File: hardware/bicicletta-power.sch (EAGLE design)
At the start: 23 parts, among them IC1 LM5017, IC2 LM1117-3.3

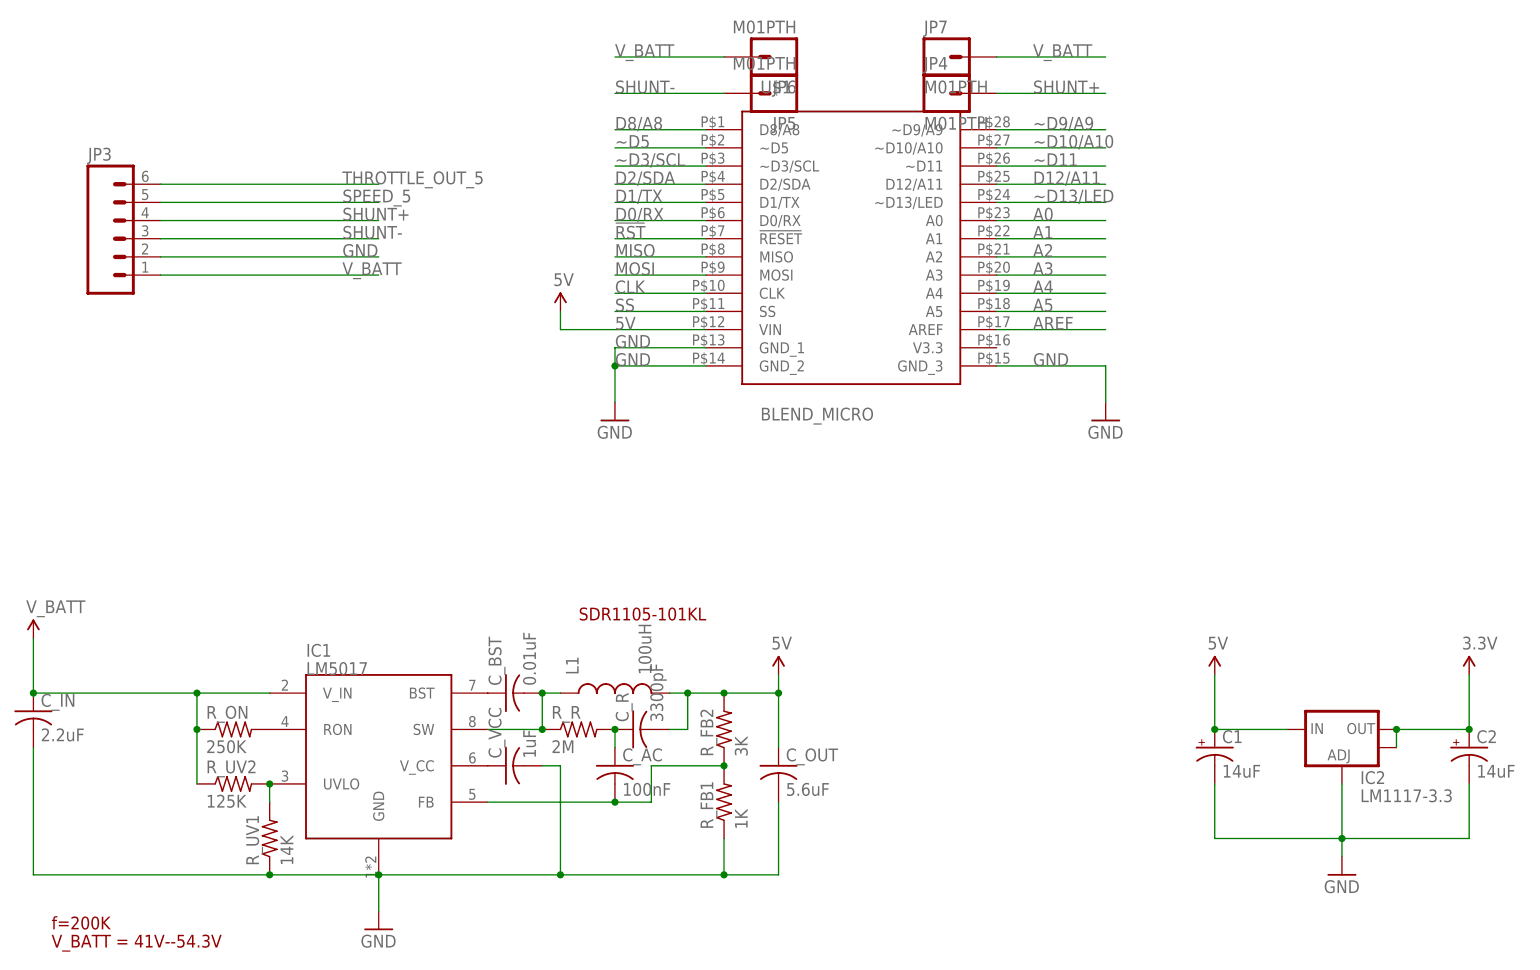
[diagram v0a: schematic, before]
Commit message: To hell with the buck regulator, let's just take 5V from the controller.
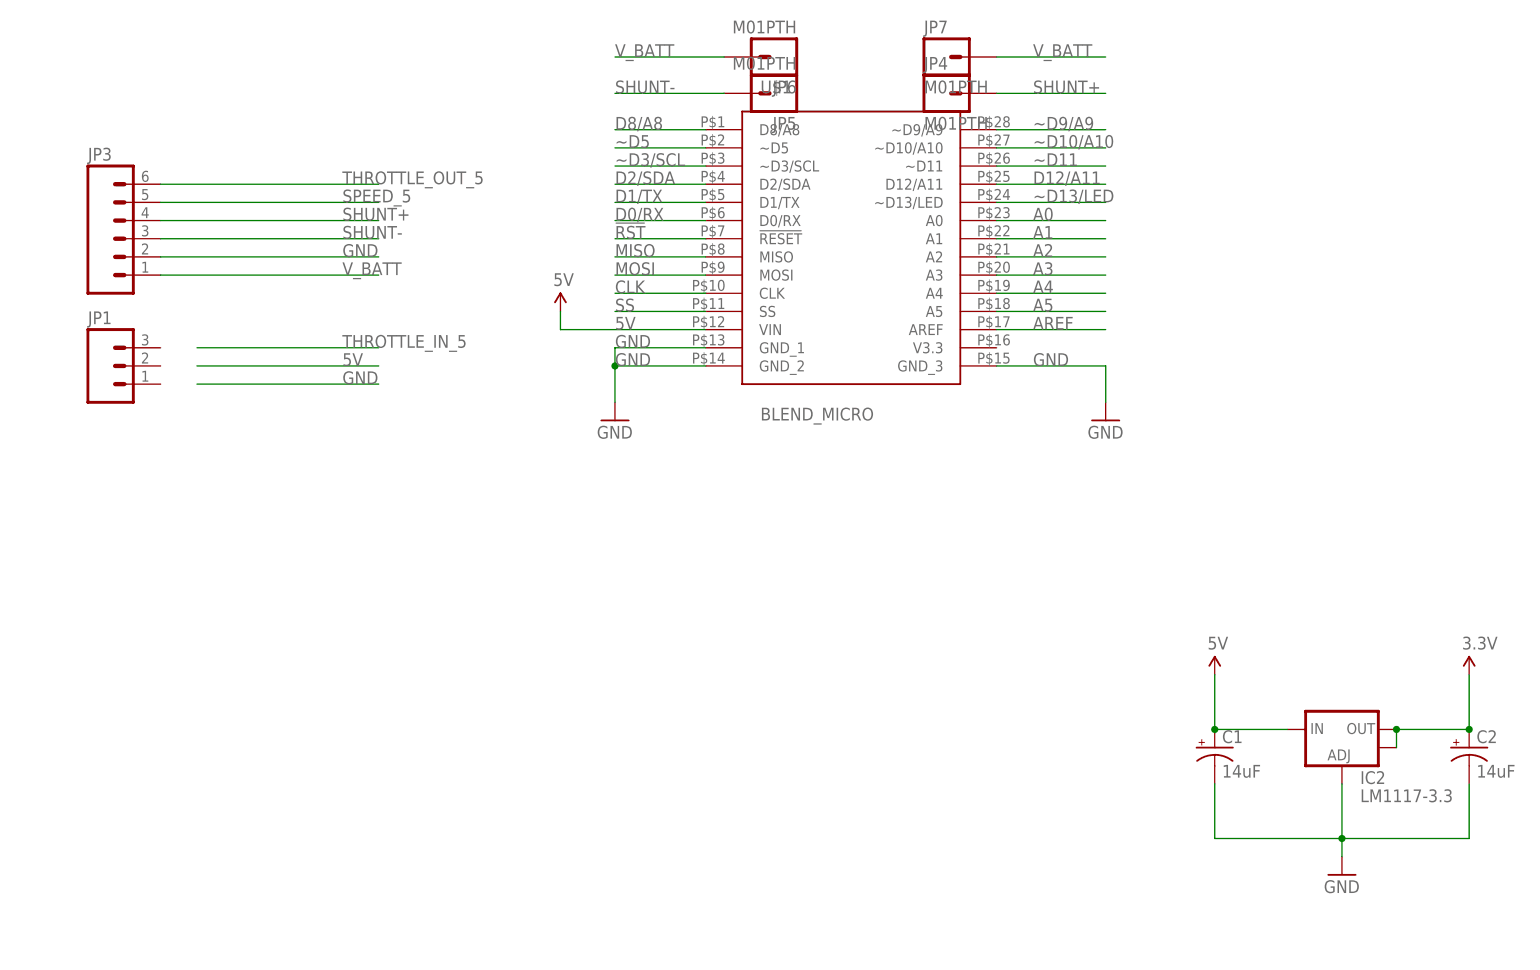
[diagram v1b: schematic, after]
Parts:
- removed C_AC: 100nF, rcl:C-USC0603
- removed C_BST: 0.01uF, rcl:C-USC0603
- removed C_IN: 2.2uF, rcl:C-USC1210K
- removed C_OUT: 5.6uF, rcl:C-USC0603
- removed C_R: 3300pF, rcl:C-USC0603
- removed C_VCC: 1uF, rcl:C-USC0603
- removed IC1: LM5017, Railstars:LM5017
- removed L1: 100uH, Railstars:SRN1060
- removed R_FB1: 1K, rcl:R-US_M0805
- removed R_FB2: 3K, rcl:R-US_M0805
- removed R_ON: 250K, rcl:R-US_M0805
- removed R_R: 2M, rcl:R-US_M0805
- removed R_UV1: 14K, rcl:R-US_M0805
- removed R_UV2: 125K, rcl:R-US_M0805
- added JP1: (no value), SparkFun-Connectors:M03PTH
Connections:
- removed net N$1: IC1.RON, R_ON.2
- removed net N$2: C_AC.2, IC1.FB, R_FB1.2, R_FB2.1
- removed net N$3: IC1.UVLO, R_UV1.2, R_UV2.2
- removed net N$4: C_BST.2, IC1.SW, L1.1, R_R.1
- removed net N$6: C_AC.1, C_R.1, R_R.2
- removed net N$7: C_BST.1, IC1.BST
- removed net N$9: C_VCC.1, IC1.V_CC
- net 5V: no longer C_OUT.1, C_R.2, L1.2, R_FB2.2
- net GND: no longer C_IN.2, C_OUT.2, C_VCC.2, IC1.GND, R_FB1.1, R_UV1.1
- net V_BATT: no longer C_IN.1, IC1.V_IN, R_ON.1, R_UV2.1
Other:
- note removed: "SDR1105-101KL"
- note removed: "V_BATT = 41V--54.3V"
- note removed: "f=200K"

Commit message: Revert "To hell with the buck regulator, let's just take 5V from the controller."
This reverts commit f16ee5c0247fff79c0027ea9109af273bc1d2e81.
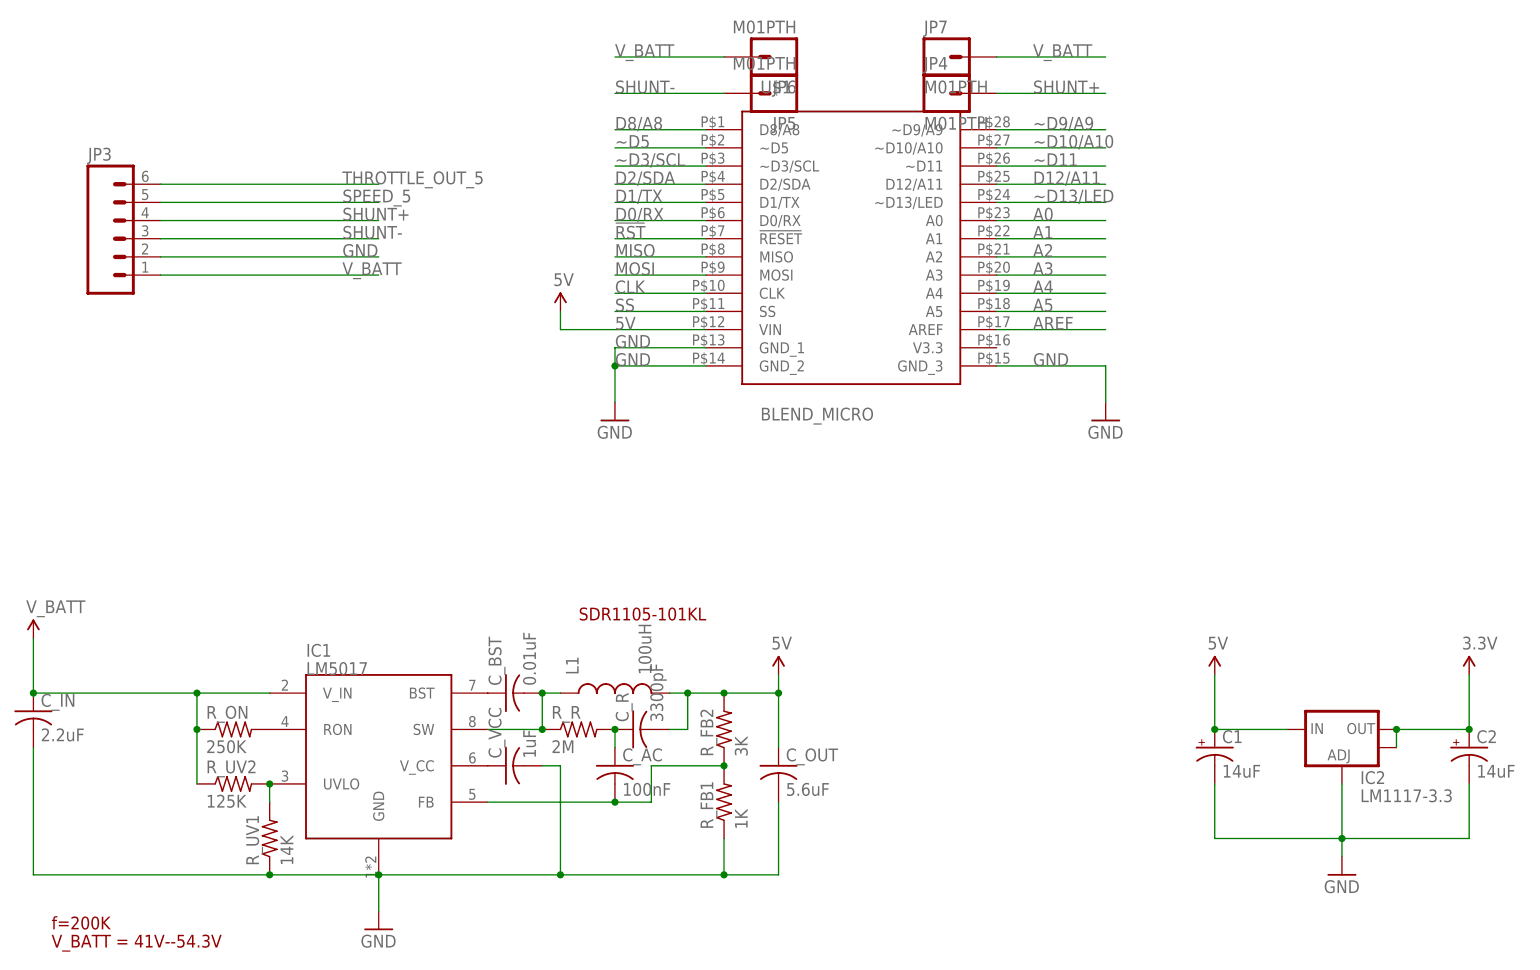
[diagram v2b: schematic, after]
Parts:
- removed JP1: (no value), SparkFun-Connectors:M03PTH
- added C_AC: 100nF, rcl:C-USC0603
- added C_BST: 0.01uF, rcl:C-USC0603
- added C_IN: 2.2uF, rcl:C-USC1210K
- added C_OUT: 5.6uF, rcl:C-USC0603
- added C_R: 3300pF, rcl:C-USC0603
- added C_VCC: 1uF, rcl:C-USC0603
- added IC1: LM5017, Railstars:LM5017
- added L1: 100uH, Railstars:SRN1060
- added R_FB1: 1K, rcl:R-US_M0805
- added R_FB2: 3K, rcl:R-US_M0805
- added R_ON: 250K, rcl:R-US_M0805
- added R_R: 2M, rcl:R-US_M0805
- added R_UV1: 14K, rcl:R-US_M0805
- added R_UV2: 125K, rcl:R-US_M0805
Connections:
- new net N$1: IC1.RON, R_ON.2
- new net N$2: C_AC.2, IC1.FB, R_FB1.2, R_FB2.1
- new net N$3: IC1.UVLO, R_UV1.2, R_UV2.2
- new net N$4: C_BST.2, IC1.SW, L1.1, R_R.1
- new net N$6: C_AC.1, C_R.1, R_R.2
- new net N$7: C_BST.1, IC1.BST
- new net N$9: C_VCC.1, IC1.V_CC
- net 5V: now also C_OUT.1, C_R.2, L1.2, R_FB2.2
- net GND: now also C_IN.2, C_OUT.2, C_VCC.2, IC1.GND, R_FB1.1, R_UV1.1
- net V_BATT: now also C_IN.1, IC1.V_IN, R_ON.1, R_UV2.1
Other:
- note added: "SDR1105-101KL"
- note added: "V_BATT = 41V--54.3V"
- note added: "f=200K"
